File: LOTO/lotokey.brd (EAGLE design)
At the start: 39.9 x 49.3 mm, 14 parts

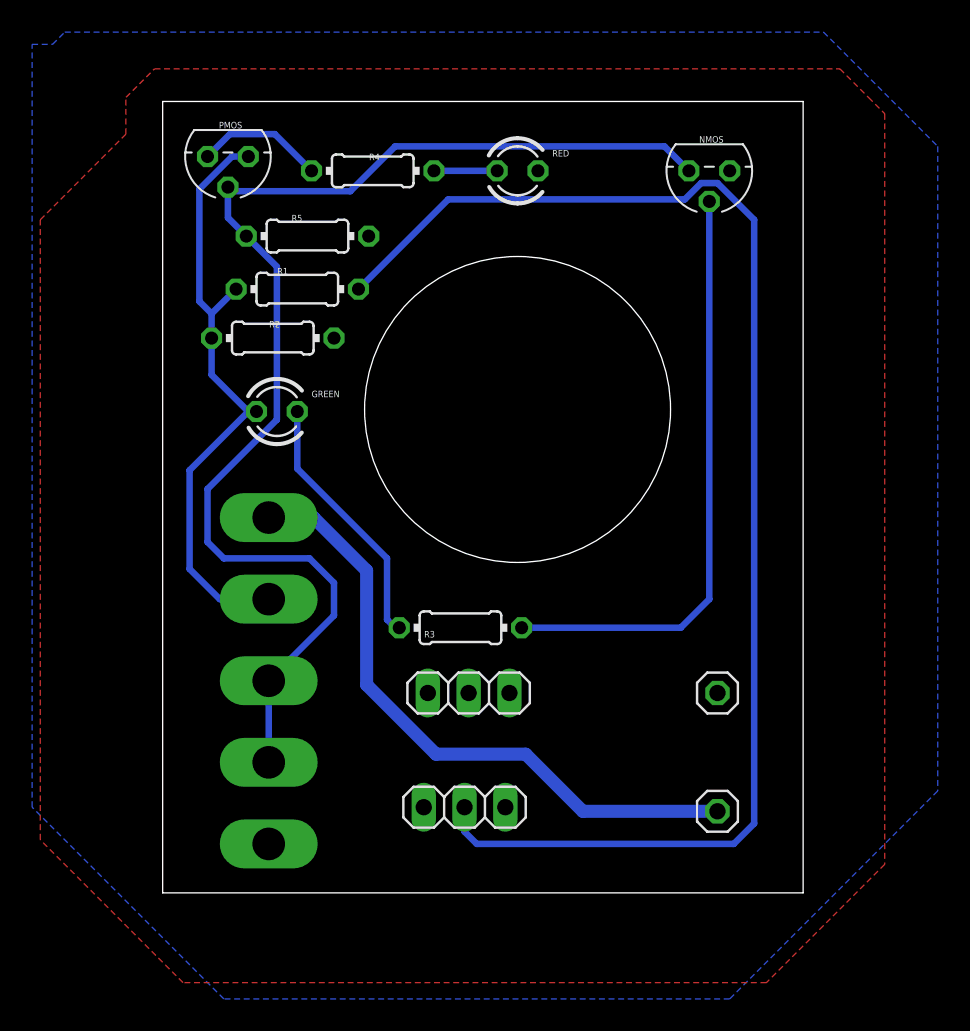
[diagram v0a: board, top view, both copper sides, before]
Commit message: adding isolated ps
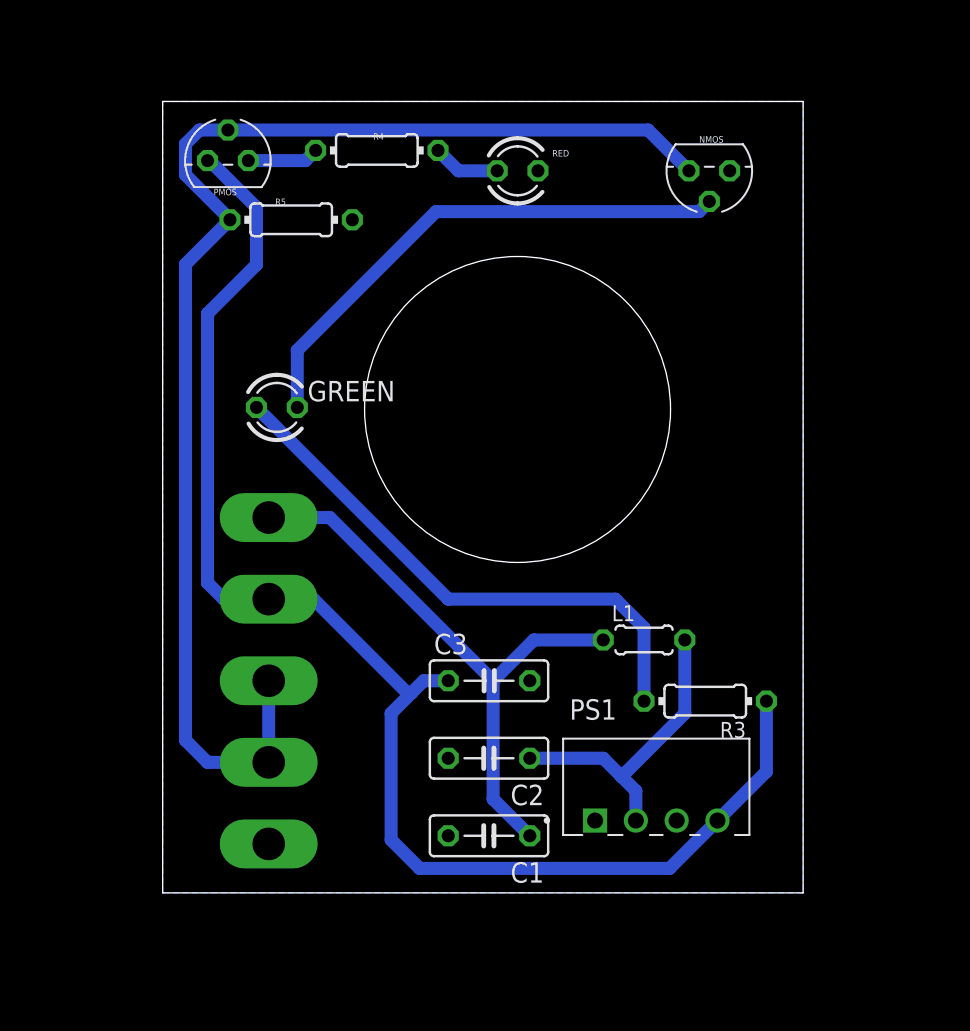
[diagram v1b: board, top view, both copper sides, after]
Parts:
- removed JP1, JP2: (no value), pinhead:1X01
- removed JP3, JP4: (no value), pinhead:1X03
- removed R1: 650, rcl:0204/7
- removed R2: 1k, rcl:0204/7
- added C1, C2: 4.7uF/25V, rcl:C050-025X075
- added C3: 10uF, rcl:C050-025X075
- added L1: (no value), rcl:0204/5
- added PS1: PDSE1-S5-S5-S, PDSE1-S5-S5-S:CONV_PDSE1-S5-S5-S
- moved R3 15.9 mm to (34.5, 12.4), turned to 180 degrees
- moved R5 1.44 mm to (8.76, 42.4)
- moved R4 1.30 mm to (14.1, 46.7)
- moved GREEN 0.25 mm to (7.87, 30.7)
- moved PMOS 0.25 mm to (4.83, 46.1), turned to 0 degrees
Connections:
- removed net N$5: NMOS.2, R3.2
- removed net VOUT_2V: JP4.2, R1.2
- new net N$1: C2.1, L1.2, PS1.2
- new net N$3: GREEN.K, NMOS.2
- net 12V: now also C1.1, L1.1; no longer JP1.1
- net GND: now also C1.2, C2.2, C3.2, PS1.1, PS1.3; no longer JP3.1, JP3.3, R2.2
- net N$4: now also GREEN.A, R3.2; no longer GREEN.K, R3.1
- net SWITCH: now also C3.1, PS1.4, R3.1; no longer GREEN.A, R1.1, R2.1
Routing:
- net VOUT_2V: track 86.3 -> 0.00 mm
- net SWITCH: track 38.7 -> 87.7 mm
- net N$5: track 37.2 -> 0.00 mm
- net N$3: track 0.00 -> 33.1 mm
- net N$1: track 0.00 -> 19.4 mm
- net N$4: track 16.2 -> 34.4 mm
- net SW_SIG: track 77.5 -> 83.0 mm
- net N$9: track 8.00 -> 4.45 mm
- net 12V: track 39.7 -> 36.7 mm
- removed copper zone on layer 1, net GND

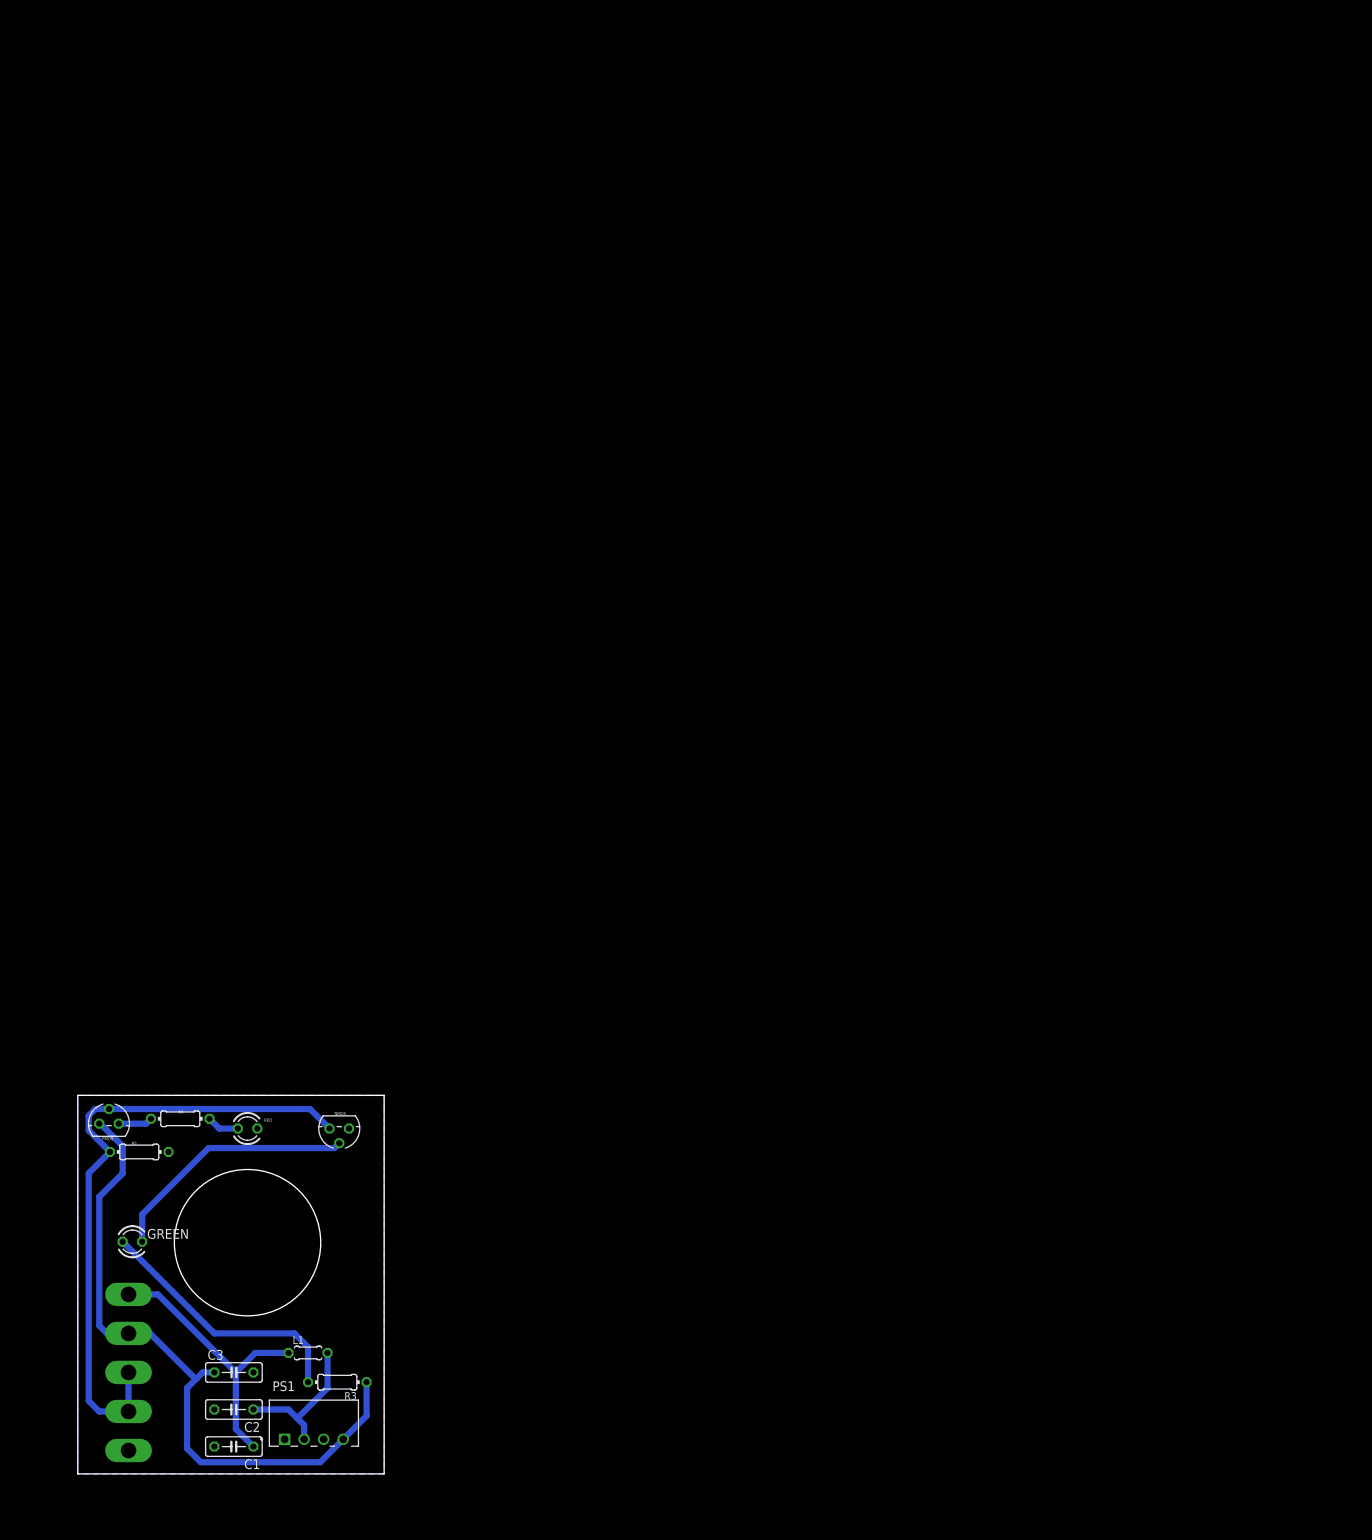
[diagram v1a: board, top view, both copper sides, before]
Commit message: Updated LOTO boards
Added LOTO housing outline.  Added logic for POE power and gate trigger. Added more circuit protection and power isolation.
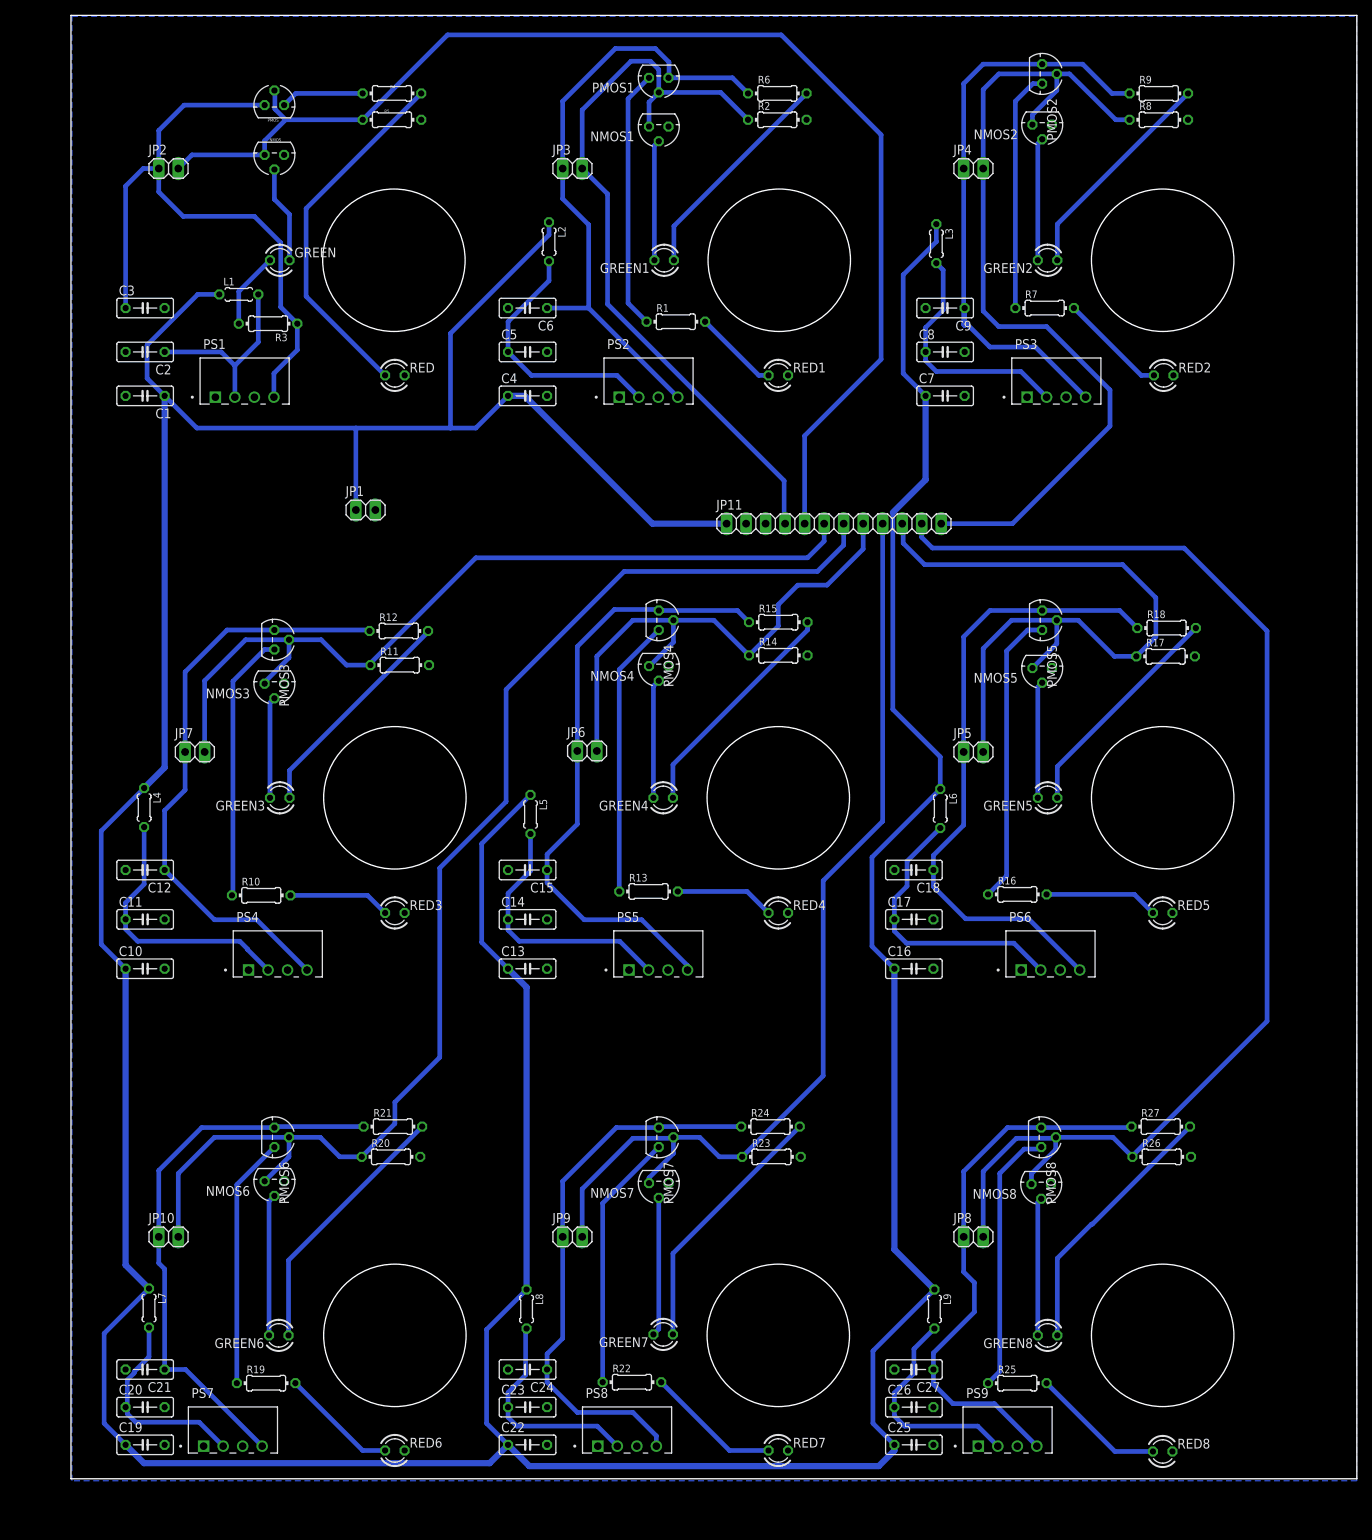
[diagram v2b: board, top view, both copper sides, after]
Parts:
- removed TERMINAL: (no value), 5mmtermblock:1X05
- added C10, C11, C13, C14, C16, C17, C19, C20, C22, C23, C25, C26, C4, C5, C7, C8: 4.7uF/25V, rcl:C050-025X075
- added C12, C15, C18, C21, C24, C27, C6, C9: 10uF, rcl:C050-025X075
- added GREEN1, GREEN2, GREEN3, GREEN4, GREEN5, GREEN6, GREEN7, GREEN8, RED1, RED2, RED3, RED4, RED5, RED6, RED7, RED8: TLLR4400, led:LED3MM
- added JP1, JP10, JP2, JP3, JP4, JP5, JP6, JP7, JP8, JP9: (no value), pinhead:1X02
- added JP11: (no value), pinhead:1X12
- added L2, L3, L4, L5, L6, L7, L8, L9: (no value), rcl:0204/5
- added NMOS1, NMOS2, NMOS3, NMOS4, NMOS5, NMOS6, NMOS7, NMOS8: BSS296, transistor-fet:TO92
- added PMOS1, PMOS2, PMOS3, PMOS4, PMOS5, PMOS6, PMOS7, PMOS8: BSS110, transistor-fet:TO92
- added PS2, PS3, PS4, PS5, PS6, PS7, PS8, PS9: PDSE1-S5-S5-S, PDSE1-S5-S5-S:CONV_PDSE1-S5-S5-S
- added R1, R10, R12, R13, R15, R16, R18, R19, R21, R22, R24, R25, R27, R6, R7, R9: 1k, rcl:0204/7
- added R11, R14, R17, R2, R20, R23, R26, R8: 10k, rcl:0204/7
- moved C3 139.0 mm to (9.53, 152.3)
- moved R5 138.3 mm to (41.7, 176.8)
- moved C2 138.2 mm to (9.53, 146.6)
- moved R3 138.1 mm to (25.5, 150.2)
- moved L1 138.1 mm to (21.7, 154.1)
- moved C1 137.3 mm to (9.53, 140.8)
- moved R4 136.3 mm to (41.7, 180.2)
- moved PS1 136.0 mm to (22.5, 142.8)
- moved PMOS 134.3 mm to (26.4, 178.7)
- moved GREEN 129.2 mm to (27.1, 158.5)
- moved NMOS 127.0 mm to (26.4, 172.2)
- moved RED 99.9 mm to (42.0, 143.5)
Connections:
- removed net 12V: C1.1, L1.1, TERMINAL.1
- removed net SWITCH: C3.1, PMOS.3, PS1.4, R3.1, TERMINAL.2
- removed net SW_SIG: NMOS.1, PMOS.2, R5.1, TERMINAL.3, TERMINAL.4
- new net +5V: C1.1, C10.1, C13.1, C16.1, C19.1, C22.1, C25.1, C4.1, C7.1, JP1.1, JP11.1, L1.1, L2.1, L3.1, L4.1, L5.1, L6.1, L7.1, L8.1, L9.1
- new net N$10: GREEN1.A, R6.2
- new net N$11: R7.2, RED2.A
- new net N$12: PMOS2.1, R7.1
- new net N$13: C8.1, L3.2, PS3.2
- new net N$14: GREEN2.K, NMOS2.2
- new net N$15: GREEN2.A, R9.2
- new net N$16: R10.2, RED3.A
- new net N$17: PMOS3.1, R10.1
- new net N$18: C11.1, L4.2, PS4.2
- new net N$19: GREEN3.K, NMOS3.2
- new net N$2: R1.2, RED1.A
- new net N$20: GREEN3.A, R12.2
- new net N$21: R13.2, RED4.A
- new net N$22: PMOS4.1, R13.1
- new net N$23: C14.1, L5.2, PS5.2
- new net N$24: GREEN4.K, NMOS4.2
- new net N$25: GREEN4.A, R15.2
- new net N$26: R16.2, RED5.A
- new net N$27: PMOS5.1, R16.1
- new net N$28: C17.1, L6.2, PS6.2
- new net N$29: GREEN5.K, NMOS5.2
- new net N$30: GREEN5.A, R18.2
- new net N$31: R19.2, RED6.A
- new net N$32: PMOS6.1, R19.1
- new net N$33: C20.1, L7.2, PS7.2
- new net N$34: GREEN6.K, NMOS6.2
- new net N$35: GREEN6.A, R21.2
- new net N$36: R22.2, RED7.A
- new net N$37: PMOS7.1, R22.1
- new net N$38: C23.1, L8.2, PS8.2
- new net N$39: GREEN7.K, NMOS7.2
- new net N$40: GREEN7.A, R24.2
- new net N$41: R25.2, RED8.A
- new net N$42: PMOS8.1, R25.1
- new net N$43: C26.1, L9.2, PS9.2
- new net N$44: GREEN8.K, NMOS8.2
- new net N$45: GREEN8.A, R27.2
- new net N$5: PMOS1.1, R1.1
- new net N$6: C5.1, L2.2, PS2.2
- new net N$7: GREEN1.K, NMOS1.2
- new net SWITCH1: C3.1, JP2.1, PMOS.3, PS1.4, R3.1
- new net SWITCH2: C6.1, JP3.1, PMOS1.3, PS2.4, R6.1
- new net SWITCH3: C9.1, JP4.1, PMOS2.3, PS3.4, R9.1
- new net SWITCH4: C18.1, JP5.1, PMOS5.3, PS6.4, R18.1
- new net SWITCH5: C15.1, JP6.1, PMOS4.3, PS5.4, R15.1
- new net SWITCH6: C12.1, JP7.1, PMOS3.3, PS4.4, R12.1
- new net SWITCH7: C27.1, JP8.1, PMOS8.3, PS9.4, R27.1
- new net SWITCH8: C24.1, JP9.1, PMOS7.3, PS8.4, R24.1
- new net SWITCH9: C21.1, JP10.1, PMOS6.3, PS7.4, R21.1
- new net SW_SIG1: JP11.5, JP2.2, NMOS.1, PMOS.2, R5.1
- new net SW_SIG2: JP11.4, JP3.2, NMOS1.1, PMOS1.2, R2.1
- new net SW_SIG3: JP11.12, JP4.2, NMOS2.1, PMOS2.2, R8.1
- new net SW_SIG4: JP11.10, JP5.2, NMOS5.1, PMOS5.2, R17.1
- new net SW_SIG5: JP11.8, JP6.2, NMOS4.1, PMOS4.2, R14.1
- new net SW_SIG6: JP11.6, JP7.2, NMOS3.1, PMOS3.2, R11.1
- new net SW_SIG7: JP11.11, JP8.2, NMOS8.1, PMOS8.2, R26.1
- new net SW_SIG8: JP11.9, JP9.2, NMOS7.1, PMOS7.2, R23.1
- new net SW_SIG9: JP10.2, JP11.7, NMOS6.1, PMOS6.2, R20.1
- net GND: now also C10.2, C11.2, C12.2, C13.2, C14.2, C15.2, C16.2, C17.2, C18.2, C19.2, C20.2, C21.2, C22.2, C23.2, C24.2, C25.2, C26.2, C27.2, C4.2, C5.2, C6.2, C7.2, C8.2, C9.2, JP1.2, JP11.2, JP11.3, NMOS1.3, NMOS2.3, NMOS3.3, NMOS4.3, NMOS5.3, NMOS6.3, NMOS7.3, NMOS8.3, PS2.1, PS2.3, PS3.1, PS3.3, PS4.1, PS4.3, PS5.1, PS5.3, PS6.1, PS6.3, PS7.1, PS7.3, PS8.1, PS8.3, PS9.1, PS9.3, R11.2, R14.2, R17.2, R2.2, R20.2, R23.2, R26.2, R8.2, RED1.K, RED2.K, RED3.K, RED4.K, RED5.K, RED6.K, RED7.K, RED8.K; no longer TERMINAL.5
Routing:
- net +5V: track 0.00 -> 667.6 mm
- net SW_SIG7: track 0.00 -> 165.7 mm
- net SW_SIG9: track 0.00 -> 165.3 mm
- net SW_SIG1: track 0.00 -> 164.3 mm
- net SW_SIG8: track 0.00 -> 128.2 mm
- net SW_SIG3: track 0.00 -> 111.8 mm
- net SW_SIG6: track 0.00 -> 109.6 mm
- net SW_SIG2: track 0.00 -> 99.3 mm
- net SW_SIG4: track 0.00 -> 91.5 mm
- net SWITCH: track 87.7 -> 0.00 mm
- net SWITCH1: track 0.00 -> 85.2 mm
- net SW_SIG: track 83.0 -> 0.00 mm
- net SWITCH4: track 0.00 -> 82.7 mm
- net SWITCH2: track 0.00 -> 80.8 mm
- net SWITCH5: track 0.00 -> 80.7 mm
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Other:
- board size 39.9 x 49.3 mm -> 167.4 x 190.5 mm
